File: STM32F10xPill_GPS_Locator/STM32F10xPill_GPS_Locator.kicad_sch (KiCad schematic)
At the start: 0 parts

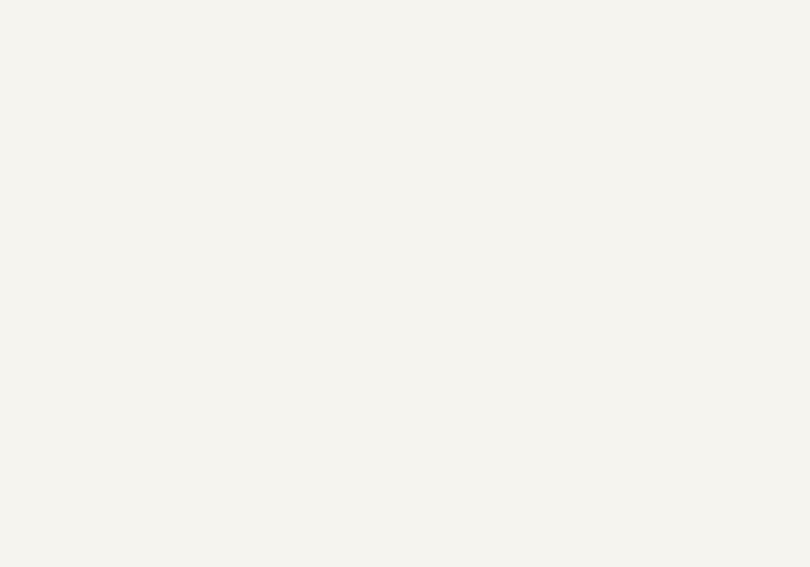
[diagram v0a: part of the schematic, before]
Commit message: Begin PCB layout
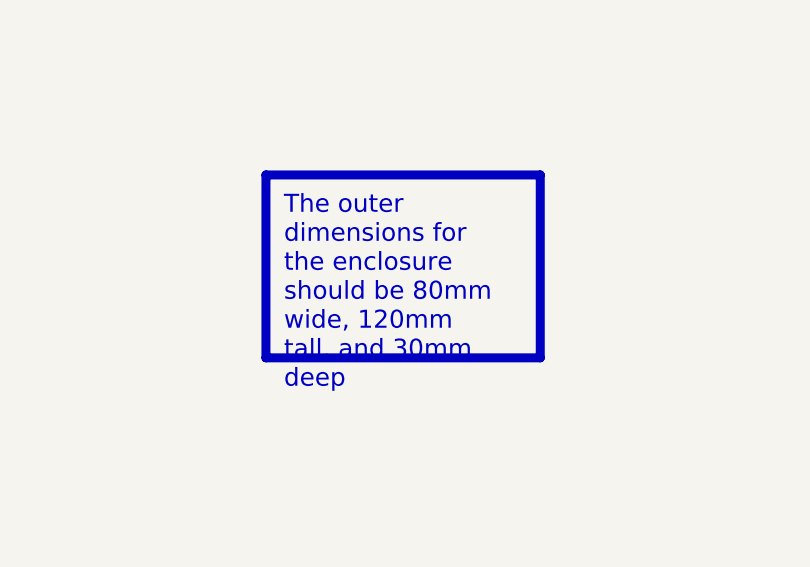
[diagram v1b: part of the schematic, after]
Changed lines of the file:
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@@
+		)
+	)
+	(text_box "The outer dimensions for the enclosure should be 80mm wide, 120mm tall, and 30mm deep"
+		(exclude_from_sim no)
+		(at 318.77 208.28 0)
+		(size 30.48 20.32)
+		(margins 2 2 2 2)
+		(stroke
+			(width 1)
+			(type solid)
+			(color 200 200 200 1)
+		)
+		(fill
+			(type none)
+		)
+		(effects
+			(font
+				(face "Arial")
+				(size 2 2)
+				(color 0 0 0 1)
+			)
+			(justify left top)
 		)
 	)
